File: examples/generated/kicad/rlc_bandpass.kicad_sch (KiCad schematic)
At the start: 5 parts

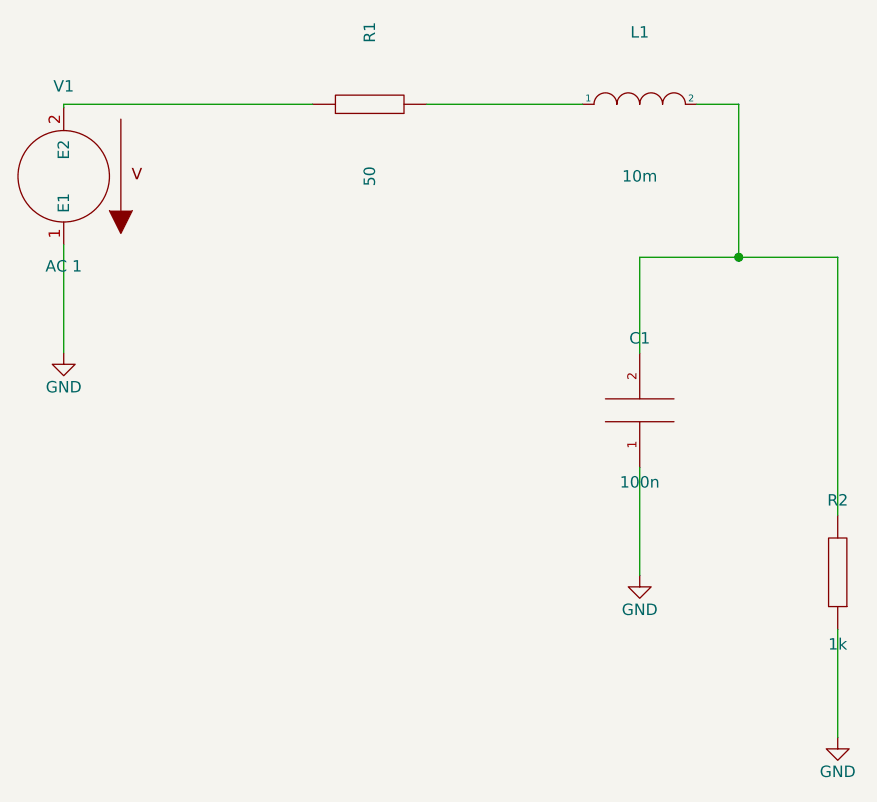
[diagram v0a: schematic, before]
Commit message: Attempt to fix more terminal issues.
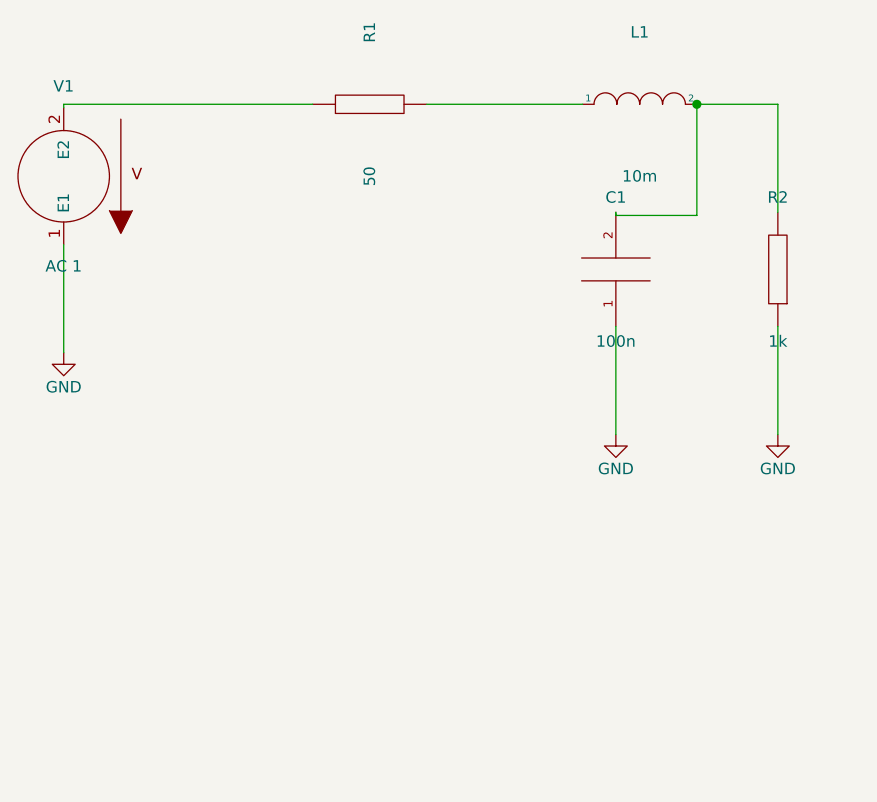
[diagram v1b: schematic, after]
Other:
- moved on the sheet: C1, R2
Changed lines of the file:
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@@
+    )
+  )
+  (symbol (lib_id "GND") (at 56.00 105.62 0) (unit 1)
+    (in_bom yes) (on_board yes)
+    (property "Reference" "#PWR0001" (at 56.0 101.81 0)
+      (effects (font (size 1.27 1.27)) hide)
+    )
+    (property "Value" "GND" (at 56.0 109.43 0)
+      (effects (font (size 1.27 1.27)))
+    )
+    (property "Footprint" "" (at 0 0 0)
+      (effects (font (size 1.27 1.27)) hide)
+    )
+    (property "Datasheet" "" (at 0 0 0)
+      (effects (font (size 1.27 1.27)) hide)
     )
   )
@@
     )
   )
-  (symbol (lib_id "CAP") (at 120.00 112.00 180) (unit 1)
+  (symbol (lib_id "CAP") (at 117.35 96.35 180) (unit 1)
     (in_bom yes) (on_board yes)
-    (property "Reference" "C1" (at 120.0 104.0 0)
+    (property "Reference" "C1" (at 117.35 88.35 0)
       (effects (font (size 1.27 1.27)))
     )
-    (property "Value" "100n" (at 120.0 120.0 0)
+    (property "Value" "100n" (at 117.35 104.35 0)
       (effects (font (size 1.27 1.27)))
     )
@@
     )
   )
-  (symbol (lib_id "R") (at 142.00 130.00 180) (unit 1)
+  (symbol (lib_id "GND") (at 117.35 114.70 0) (unit 1)
     (in_bom yes) (on_board yes)
-    (property "Reference" "R2" (at 142.0 122.0 0)
-      (effects (font (size 1.27 1.27)))
+    (property "Reference" "#PWR0002" (at 117.35 110.89 0)
+      (effects (font (size 1.27 1.27)) hide)
     )
-    (property "Value" "1k" (at 142.0 138.0 0)
+    (property "Value" "GND" (at 117.35 118.51 0)
       (effects (font (size 1.27 1.27)))
     )
@@
     )
   )
-  (symbol (lib_id "GND") (at 56.00 105.62 0) (unit 1)
+  (symbol (lib_id "R") (at 135.35 96.35 180) (unit 1)
     (in_bom yes) (on_board yes)
-    (property "Reference" "#PWR0001" (at 56.0 101.81 0)
-      (effects (font (size 1.27 1.27)) hide)
+    (property "Reference" "R2" (at 135.35 88.35 0)
+      (effects (font (size 1.27 1.27)))
     )
-    (property "Value" "GND" (at 56.0 109.43 0)
+    (property "Value" "1k" (at 135.35 104.35 0)
       (effects (font (size 1.27 1.27)))
     )
@@
     )
   )
-  (symbol (lib_id "GND") (at 120.00 130.35 0) (unit 1)
+  (symbol (lib_id "GND") (at 135.35 114.70 0) (unit 1)
     (in_bom yes) (on_board yes)
-    (property "Reference" "#PWR0002" (at 120.0 126.53999999999999 0)
+    (property "Reference" "#PWR0003" (at 135.35 110.89 0)
       (effects (font (size 1.27 1.27)) hide)
     )
-    (property "Value" "GND" (at 120.0 134.16 0)
+    (property "Value" "GND" (at 135.35 118.51 0)
       (effects (font (size 1.27 1.27)))
     )
@@
     )
   )
-  (symbol (lib_id "GND") (at 142.00 148.35 0) (unit 1)
-    (in_bom yes) (on_board yes)
-    (property "Reference" "#PWR0003" (at 142.0 144.54 0)
-      (effects (font (size 1.27 1.27)) hide)
-    )
-    (property "Value" "GND" (at 142.0 152.16 0)
-      (effects (font (size 1.27 1.27)))
-    )
-    (property "Footprint" "" (at 0 0 0)
-      (effects (font (size 1.27 1.27)) hide)
-    )
-    (property "Datasheet" "" (at 0 0 0)
-      (effects (font (size 1.27 1.27)) hide)
-    )
+  (wire (pts (xy 117.35 102.70) (xy 117.35 114.70))
+    (stroke (width 0) (type solid) (color 0 0 0 0))
+  )
+  (wire (pts (xy 135.35 102.70) (xy 135.35 114.70))
+    (stroke (width 0) (type solid) (color 0 0 0 0))
   )
   (wire (pts (xy 56.00 93.62) (xy 56.00 105.62))
-    (stroke (width 0) (type solid) (color 0 0 0 0))
-  )
-  (wire (pts (xy 120.00 118.35) (xy 120.00 130.35))
-    (stroke (width 0) (type solid) (color 0 0 0 0))
-  )
-  (wire (pts (xy 142.00 136.35) (xy 142.00 148.35))
-    (stroke (width 0) (type solid) (color 0 0 0 0))
-  )
-  (wire (pts (xy 96.35 78.00) (xy 113.65 78.00))
-    (stroke (width 0) (type solid) (color 0 0 0 0))
-  )
-  (wire (pts (xy 126.35 78.00) (xy 131.00 78.00))
-    (stroke (width 0) (type solid) (color 0 0 0 0))
-  )
-  (wire (pts (xy 131.00 78.00) (xy 131.00 95.00))
-    (stroke (width 0) (type solid) (color 0 0 0 0))
-  )
-  (wire (pts (xy 120.00 105.65) (xy 120.00 95.00))
-    (stroke (width 0) (type solid) (color 0 0 0 0))
-  )
-  (wire (pts (xy 120.00 95.00) (xy 131.00 95.00))
-    (stroke (width 0) (type solid) (color 0 0 0 0))
-  )
-  (wire (pts (xy 142.00 123.65) (xy 142.00 95.00))
-    (stroke (width 0) (type solid) (color 0 0 0 0))
-  )
-  (wire (pts (xy 142.00 95.00) (xy 131.00 95.00))
     (stroke (width 0) (type solid) (color 0 0 0 0))
   )
@@
     (stroke (width 0) (type solid) (color 0 0 0 0))
   )
-  (junction (at 131.00 95.00) (diameter 1.016) (color 0 0 0 0))
+  (wire (pts (xy 96.35 78.00) (xy 113.65 78.00))
+    (stroke (width 0) (type solid) (color 0 0 0 0))
+  )
+  (wire (pts (xy 117.35 90.00) (xy 117.35 90.35))
+    (stroke (width 0) (type solid) (color 0 0 0 0))
+  )
+  (wire (pts (xy 117.35 90.35) (xy 126.35 90.35))
+    (stroke (width 0) (type solid) (color 0 0 0 0))
+  )
+  (wire (pts (xy 126.35 90.35) (xy 126.35 78.00))
+    (stroke (width 0) (type solid) (color 0 0 0 0))
+  )
+  (wire (pts (xy 135.35 90.00) (xy 135.35 78.00))
+    (stroke (width 0) (type solid) (color 0 0 0 0))
+  )
+  (wire (pts (xy 135.35 78.00) (xy 126.35 78.00))
+    (stroke (width 0) (type solid) (color 0 0 0 0))
+  )
+  (junction (at 126.35 78.00) (diameter 1.016) (color 0 0 0 0))
   (sheet_instances
     (path "/" (page "1"))
@@
   (symbol_instances
     (path "/ff7a382b-150d-5dda-af7d-43696bfc33d8" (reference "V1") (unit 1) (value "AC 1") (footprint ""))
+    (path "/377a3052-07db-5d7e-aabd-1d809c76f718" (reference "#PWR0001") (unit 1) (value "GND") (footprint ""))
     (path "/2d26d2d6-68a6-5166-92c8-b235f4198e44" (reference "R1") (unit 1) (value "50") (footprint ""))
     (path "/d51770c5-9dd4-52f2-beba-2e847cdaa82c" (reference "L1") (unit 1) (value "10m") (footprint ""))
     (path "/cd1f9510-5b53-5cd9-9b95-17115dad0ad7" (reference "C1") (unit 1) (value "100n") (footprint ""))
+    (path "/73773ef2-52e2-515f-9193-ba4c4c232fbe" (reference "#PWR0002") (unit 1) (value "GND") (footprint ""))
     (path "/b1d9c617-2a8f-5ec8-b477-3e4c80c09fda" (reference "R2") (unit 1) (value "1k") (footprint ""))
-    (path "/377a3052-07db-5d7e-aabd-1d809c76f718" (reference "#PWR0001") (unit 1) (value "GND") (footprint ""))
-    (path "/73773ef2-52e2-515f-9193-ba4c4c232fbe" (reference "#PWR0002") (unit 1) (value "GND") (footprint ""))
     (path "/031d87f3-084d-5a64-83f1-7b1a54b82eb9" (reference "#PWR0003") (unit 1) (value "GND") (footprint ""))
   )
